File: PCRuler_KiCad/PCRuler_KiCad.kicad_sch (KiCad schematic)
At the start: 30 parts, among them Q1 DMMT5401, SW1 CK_KMS2xxG, SW2 CK_KMS2xxG, U1 ICM7555xB, U2 ATmega8-16A, U3 PAM8406D, Y1 Crystal

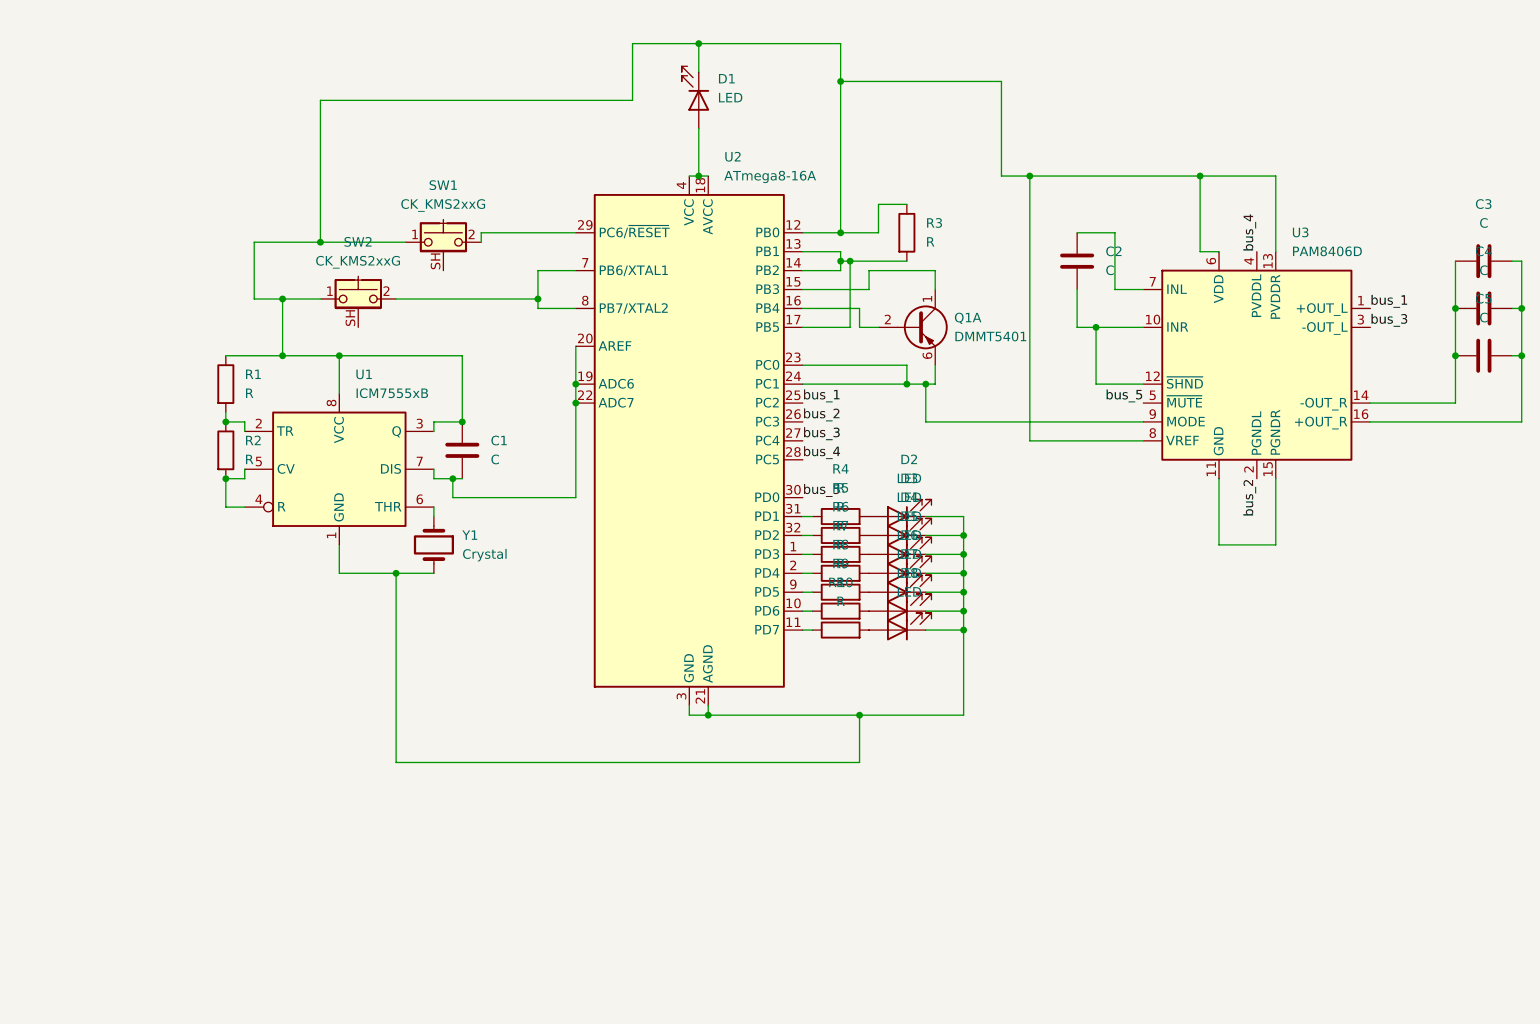
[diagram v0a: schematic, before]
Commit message: Re-did almost everything
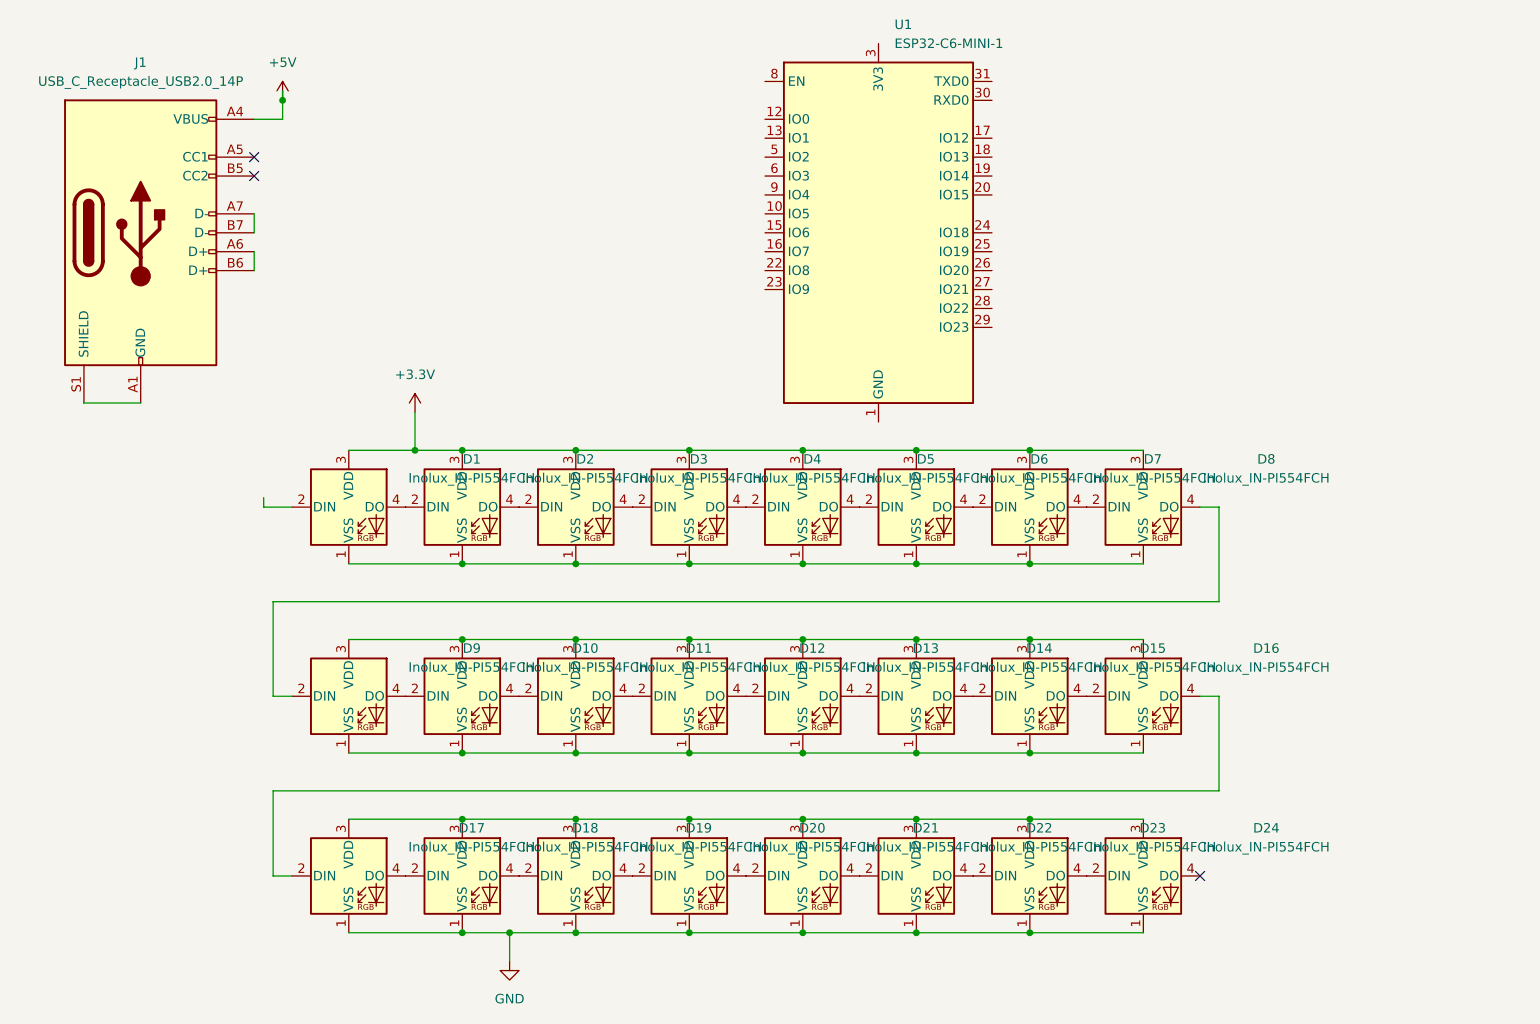
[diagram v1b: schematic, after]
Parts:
- removed C1, C2, C3, C4, C5: C, Capacitor_SMD:C_1812_4532Metric, symbol Device:C
- removed D1, D2, D3, D4, D5, D6, D7, D8: LED, LED_SMD:LED_0805_2012Metric, symbol Device:LED
- removed Q1: DMMT5401, Package_TO_SOT_SMD:SOT-23-6, symbol Transistor_BJT:DMMT5401
- removed R1, R10, R2, R3, R4, R5, R6, R7, R8, R9: R, Resistor_SMD:R_0402_1005Metric, symbol Device:R
- removed SW1, SW2: CK_KMS2xxG, Button_Switch_SMD:SW_SPST_CK_KMS2xxGP, symbol Switch:CK_KMS2xxG
- removed U1: ICM7555xB, Package_SO:SOIC-8_3.9x4.9mm_P1.27mm, symbol Timer:ICM7555xB
- removed U2: ATmega8-16A, Package_QFP:TQFP-32_7x7mm_P0.8mm, symbol MCU_Microchip_ATmega:ATmega8-16A
- removed U3: PAM8406D, Package_SO:SOIC-16_3.9x9.9mm_P1.27mm, symbol Amplifier_Audio:PAM8406D
- removed Y1: Crystal, Crystal:Crystal_SMD_0603-4Pin_6.0x3.5mm, symbol Device:Crystal
- added D1, D10, D11, D12, D13, D14, D15, D16, D17, D18, D19, D2, D20, D21, D22, D23, D24, D3, D4, D5, D6, D7, D8, D9: Inolux_IN-PI554FCH, LED_SMD:LED_Inolux_IN-PI554FCH_PLCC4_5.0x5.0mm_P3.2mm, symbol LED:Inolux_IN-PI554FCH
- added J1: USB_C_Receptacle_USB2.0_14P, symbol Connector:USB_C_Receptacle_USB2.0_14P
- added U1: ESP32-C6-MINI-1, RF_Module:ESP32-C6-MINI-1, symbol RF_Module:ESP32-C6-MINI-1
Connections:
- new net: D22.4 (DO), D23.2 (DIN)
- new net: D17.3 (VDD), D18.3 (VDD), D19.3 (VDD), D20.3 (VDD), D21.3 (VDD), D22.3 (VDD), D23.3 (VDD), D24.3 (VDD)
- new net: D23.4 (DO), D24.2 (DIN)
- new net: D18.4 (DO), D19.2 (DIN)
- new net: D19.4 (DO), D20.2 (DIN)
- new net: D1.1 (VSS), D2.1 (VSS), D3.1 (VSS), D4.1 (VSS), D5.1 (VSS), D6.1 (VSS), D7.1 (VSS), D8.1 (VSS)
- new net: D1.4 (DO), D2.2 (DIN)
- new net: D2.4 (DO), D3.2 (DIN)
- new net: D21.4 (DO), D22.2 (DIN)
- new net: D20.4 (DO), D21.2 (DIN)
- new net: D7.4 (DO), D8.2 (DIN)
- new net: D8.4 (DO), D9.2 (DIN)
- new net: D3.4 (DO), D4.2 (DIN)
- new net: D4.4 (DO), D5.2 (DIN)
- new net: J1.A1 (GND), J1.A12 (GND), J1.B1 (GND), J1.B12 (GND), J1.S1 (SHIELD)
- new net: J1.A6 (D+), J1.B6 (D+)
- new net: J1.A7 (D-), J1.B7 (D-)
- new net: D6.4 (DO), D7.2 (DIN)
- new net: D17.4 (DO), D18.2 (DIN)
- new net: D10.1 (VSS), D11.1 (VSS), D12.1 (VSS), D13.1 (VSS), D14.1 (VSS), D15.1 (VSS), D16.1 (VSS), D9.1 (VSS)
- new net: D13.4 (DO), D14.2 (DIN)
- new net: D10.3 (VDD), D11.3 (VDD), D12.3 (VDD), D13.3 (VDD), D14.3 (VDD), D15.3 (VDD), D16.3 (VDD), D9.3 (VDD)
- new net: D14.4 (DO), D15.2 (DIN)
- new net: D10.2 (DIN), D9.4 (DO)
- new net: D5.4 (DO), D6.2 (DIN)
- new net: D15.4 (DO), D16.2 (DIN)
- new net: D12.4 (DO), D13.2 (DIN)
- new net: D10.4 (DO), D11.2 (DIN)
- new net: D11.4 (DO), D12.2 (DIN)
- new net: U1.1 (GND), U1.11 (GND), U1.14 (GND), U1.2 (GND), U1.36 (GND), U1.37 (GND), U1.38 (GND), U1.39 (GND), U1.40 (GND), U1.41 (GND), U1.42 (GND), U1.43 (GND), U1.44 (GND), U1.45 (GND), U1.46 (GND), U1.47 (GND), U1.48 (GND), U1.49 (GND), U1.50 (GND), U1.51 (GND), U1.52 (GND), U1.53 (GND)
- new net: D16.4 (DO), D17.2 (DIN)
- new net +3.3V: D1.3 (VDD), D2.3 (VDD), D3.3 (VDD), D4.3 (VDD), D5.3 (VDD), D6.3 (VDD), D7.3 (VDD), D8.3 (VDD)
- new net +5V: J1.A4 (VBUS), J1.A9 (VBUS), J1.B4 (VBUS), J1.B9 (VBUS)
- new net GND: D17.1 (VSS), D18.1 (VSS), D19.1 (VSS), D20.1 (VSS), D21.1 (VSS), D22.1 (VSS), D23.1 (VSS), D24.1 (VSS)
- no-connect marks 0 -> 3
